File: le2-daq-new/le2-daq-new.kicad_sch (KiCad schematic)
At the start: 10 parts, among them J1 PCIE_CONN, J2 PCIE_CONN, J3 PCIE_CONN, J4 PCIE_CONN, J5 Conn_01x02_Male, J6 TEST-POINT, J7 TEST-POINT, SW1 SW_Push, U1 ESP32-DEVKITC-32D

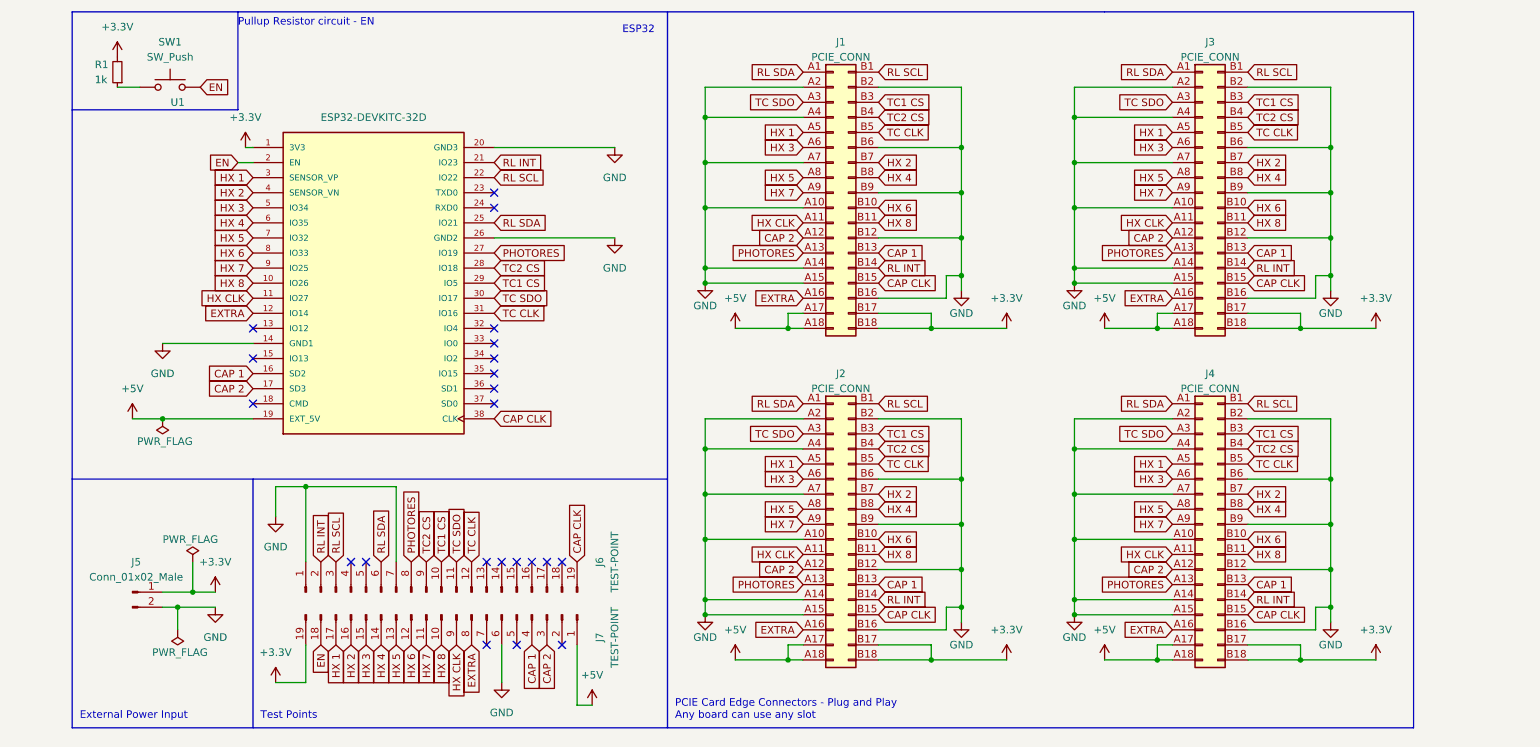
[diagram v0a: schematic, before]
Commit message: done with daq layout FRFRFRF
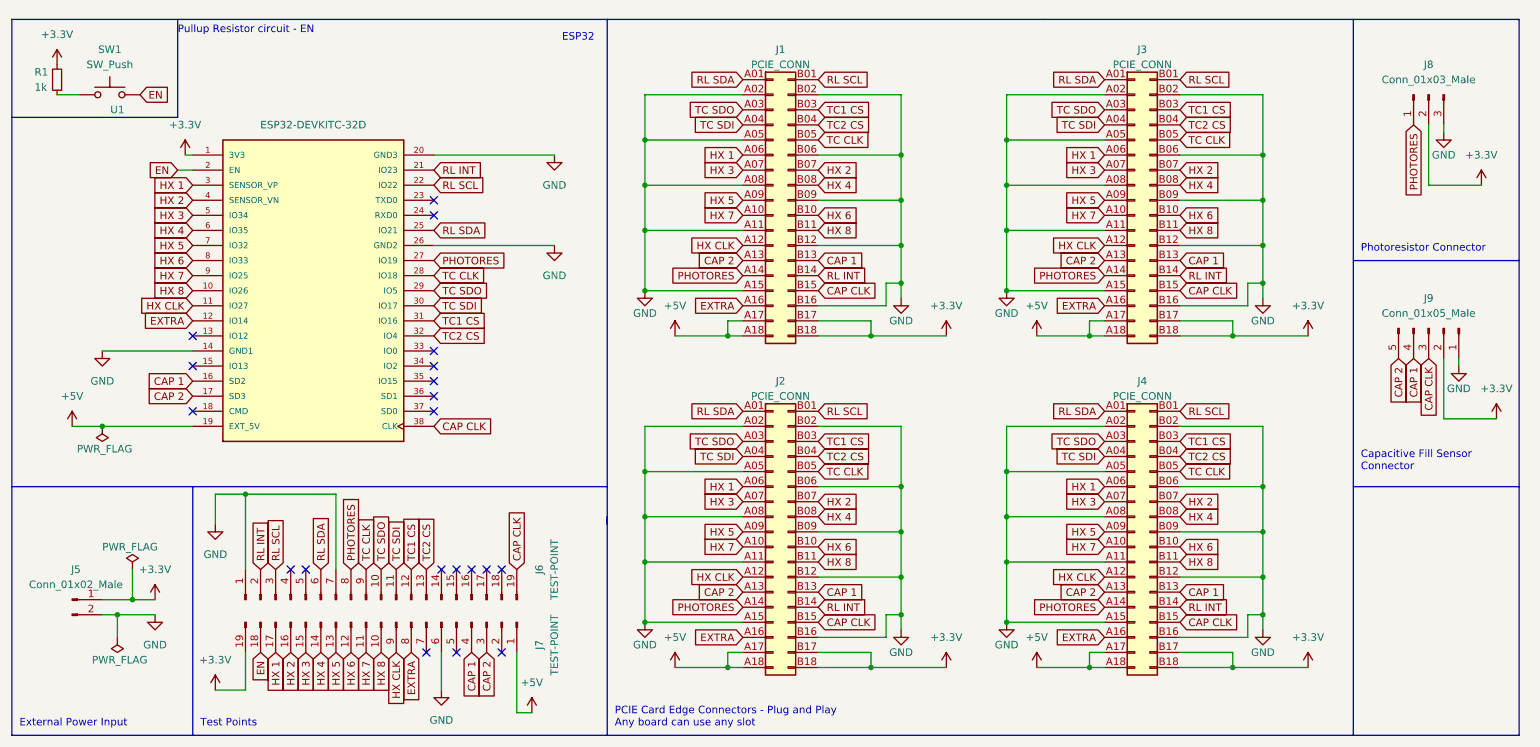
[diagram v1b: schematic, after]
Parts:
- added J8: Conn_01x03_Male, Connector_PinHeader_2.54mm:PinHeader_1x03_P2.54mm_Vertical, symbol Connector:Conn_01x03_Male
- added J9: Conn_01x05_Male, Connector_PinHeader_2.54mm:PinHeader_1x05_P2.54mm_Vertical, symbol Connector:Conn_01x05_Male
- J1, J2, J3, J4: footprint PCIE-LP-01-01-F-DV-A-TR:SAMTEC_PCIE-LP-01-01-F-DV-A-TR -> AMPHENOL-PCIE-Socket:AMPHENOL_10018784-10210TLF
- J5: footprint Connector_PinHeader_2.54mm:PinHeader_1x02_P2.54mm_Horizontal -> Connector_PinHeader_2.54mm:PinHeader_1x02_P2.54mm_Vertical
- J6, J7: footprint Connector_PinHeader_2.54mm:PinHeader_1x19_P2.54mm_Horizontal -> Connector_PinHeader_2.54mm:PinHeader_1x19_P2.54mm_Vertical
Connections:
- net +3.3V: now also J8.2 (Pin_2), J9.2 (Pin_2)
- net CAP 1: now also J9.4 (Pin_4)
- net CAP 2: now also J1.A13 (Pin_a13), J2.A13 (Pin_a13), J3.A13 (Pin_a13), J4.A13 (Pin_a13), J9.5 (Pin_5); no longer J1.A12 (Pin_a12), J2.A12 (Pin_a12), J3.A12 (Pin_a12), J4.A12 (Pin_a12)
- net CAP CLK: now also J9.3 (Pin_3)
- net GND: now also J1.A02 (Pin_a2), J1.A05 (Pin_a5), J1.A08 (Pin_a8), J1.A11 (Pin_a11), J1.B02 (Pin_b2), J1.B06 (Pin_b6), J1.B09 (Pin_b9), J2.A02 (Pin_a2), J2.A05 (Pin_a5), J2.A08 (Pin_a8), J2.A11 (Pin_a11), J2.B02 (Pin_b2), J2.B06 (Pin_b6), J2.B09 (Pin_b9), J3.A02 (Pin_a2), J3.A05 (Pin_a5), J3.A08 (Pin_a8), J3.A11 (Pin_a11), J3.B02 (Pin_b2), J3.B06 (Pin_b6), J3.B09 (Pin_b9), J4.A02 (Pin_a2), J4.A05 (Pin_a5), J4.A08 (Pin_a8), J4.A11 (Pin_a11), J4.B02 (Pin_b2), J4.B06 (Pin_b6), J4.B09 (Pin_b9), J8.3 (Pin_3), J9.1 (Pin_1); no longer J1.A10 (Pin_a10), J1.A14 (Pin_a14), J1.A2 (Pin_a2), J1.A4 (Pin_a4), J1.A7 (Pin_a7), J1.B2 (Pin_b2), J1.B6 (Pin_b6), J1.B9 (Pin_b9), J2.A10 (Pin_a10), J2.A14 (Pin_a14), J2.A2 (Pin_a2), J2.A4 (Pin_a4), J2.A7 (Pin_a7), J2.B2 (Pin_b2), J2.B6 (Pin_b6), J2.B9 (Pin_b9), J3.A10 (Pin_a10), J3.A14 (Pin_a14), J3.A2 (Pin_a2), J3.A4 (Pin_a4), J3.A7 (Pin_a7), J3.B2 (Pin_b2), J3.B6 (Pin_b6), J3.B9 (Pin_b9), J4.A10 (Pin_a10), J4.A14 (Pin_a14), J4.A2 (Pin_a2), J4.A4 (Pin_a4), J4.A7 (Pin_a7), J4.B2 (Pin_b2), J4.B6 (Pin_b6), J4.B9 (Pin_b9)
- net HX 1: now also J1.A06 (Pin_a6), J2.A06 (Pin_a6), J3.A06 (Pin_a6), J4.A06 (Pin_a6); no longer J1.A5 (Pin_a5), J2.A5 (Pin_a5), J3.A5 (Pin_a5), J4.A5 (Pin_a5)
- net HX 2: now also J1.B07 (Pin_b7), J2.B07 (Pin_b7), J3.B07 (Pin_b7), J4.B07 (Pin_b7); no longer J1.B7 (Pin_b7), J2.B7 (Pin_b7), J3.B7 (Pin_b7), J4.B7 (Pin_b7)
- net HX 3: now also J1.A07 (Pin_a7), J2.A07 (Pin_a7), J3.A07 (Pin_a7), J4.A07 (Pin_a7); no longer J1.A6 (Pin_a6), J2.A6 (Pin_a6), J3.A6 (Pin_a6), J4.A6 (Pin_a6)
- net HX 4: now also J1.B08 (Pin_b8), J2.B08 (Pin_b8), J3.B08 (Pin_b8), J4.B08 (Pin_b8); no longer J1.B8 (Pin_b8), J2.B8 (Pin_b8), J3.B8 (Pin_b8), J4.B8 (Pin_b8)
- net HX 5: now also J1.A09 (Pin_a9), J2.A09 (Pin_a9), J3.A09 (Pin_a9), J4.A09 (Pin_a9); no longer J1.A8 (Pin_a8), J2.A8 (Pin_a8), J3.A8 (Pin_a8), J4.A8 (Pin_a8)
- net HX 7: now also J1.A10 (Pin_a10), J2.A10 (Pin_a10), J3.A10 (Pin_a10), J4.A10 (Pin_a10); no longer J1.A9 (Pin_a9), J2.A9 (Pin_a9), J3.A9 (Pin_a9), J4.A9 (Pin_a9)
- net HX CLK: now also J1.A12 (Pin_a12), J2.A12 (Pin_a12), J3.A12 (Pin_a12), J4.A12 (Pin_a12); no longer J1.A11 (Pin_a11), J2.A11 (Pin_a11), J3.A11 (Pin_a11), J4.A11 (Pin_a11)
- net PHOTORES: now also J1.A14 (Pin_a14), J2.A14 (Pin_a14), J3.A14 (Pin_a14), J4.A14 (Pin_a14), J8.1 (Pin_1); no longer J1.A13 (Pin_a13), J2.A13 (Pin_a13), J3.A13 (Pin_a13), J4.A13 (Pin_a13)
- net RL SCL: now also J1.B01 (Pin_b1), J2.B01 (Pin_b1), J3.B01 (Pin_b1), J4.B01 (Pin_b1); no longer J1.B1 (Pin_b1), J2.B1 (Pin_b1), J3.B1 (Pin_b1), J4.B1 (Pin_b1)
- net RL SDA: now also J1.A01 (Pin_a1), J2.A01 (Pin_a1), J3.A01 (Pin_a1), J4.A01 (Pin_a1); no longer J1.A1 (Pin_a1), J2.A1 (Pin_a1), J3.A1 (Pin_a1), J4.A1 (Pin_a1)
- net TC CLK: now also J1.B05 (Pin_b5), J2.B05 (Pin_b5), J3.B05 (Pin_b5), J4.B05 (Pin_b5), J6.9 (Pin_9), U1.28 (IO18); no longer J1.B5 (Pin_b5), J2.B5 (Pin_b5), J3.B5 (Pin_b5), J4.B5 (Pin_b5), J6.12 (Pin_12), U1.31 (IO16)
- net TC SDO: now also J1.A03 (Pin_a3), J2.A03 (Pin_a3), J3.A03 (Pin_a3), J4.A03 (Pin_a3), J6.10 (Pin_10), U1.29 (IO5); no longer J1.A3 (Pin_a3), J2.A3 (Pin_a3), J3.A3 (Pin_a3), J4.A3 (Pin_a3), J6.11 (Pin_11), U1.30 (IO17)
- net TC1 CS: now also J1.B03 (Pin_b3), J2.B03 (Pin_b3), J3.B03 (Pin_b3), J4.B03 (Pin_b3), J6.12 (Pin_12), U1.31 (IO16); no longer J1.B3 (Pin_b3), J2.B3 (Pin_b3), J3.B3 (Pin_b3), J4.B3 (Pin_b3), J6.10 (Pin_10), U1.29 (IO5)
- net TC2 CS: now also J1.B04 (Pin_b4), J2.B04 (Pin_b4), J3.B04 (Pin_b4), J4.B04 (Pin_b4), J6.13 (Pin_13), U1.32 (IO4); no longer J1.B4 (Pin_b4), J2.B4 (Pin_b4), J3.B4 (Pin_b4), J4.B4 (Pin_b4), J6.9 (Pin_9), U1.28 (IO18)
- new net TC SDI: J1.A04 (Pin_a4), J2.A04 (Pin_a4), J3.A04 (Pin_a4), J4.A04 (Pin_a4), J6.11 (Pin_11), U1.30 (IO17)
- no-connect marks 22 -> 20
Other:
- note added: "Capacitive Fill Sensor Connector"
- note added: "Photoresistor Connector"
- moved on the sheet: J1, J5, J6, J7, R1, SW1, U1
